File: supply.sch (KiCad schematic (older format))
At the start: 44 parts, among them IC1 MIC5317-2.5YM5-TR, J1 WE_629105150521, U1 FT2232HL-REEL, Y1 KX-7_12,MHz

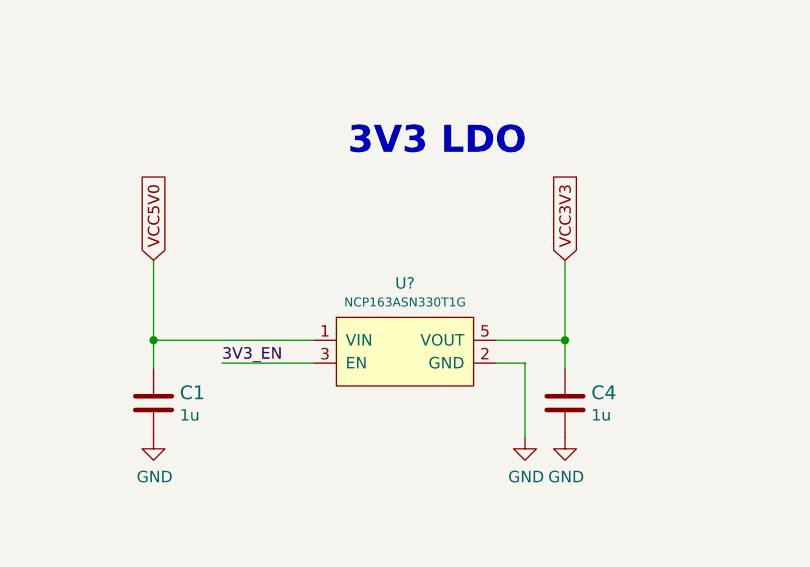
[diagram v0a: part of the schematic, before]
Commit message: Annotate components
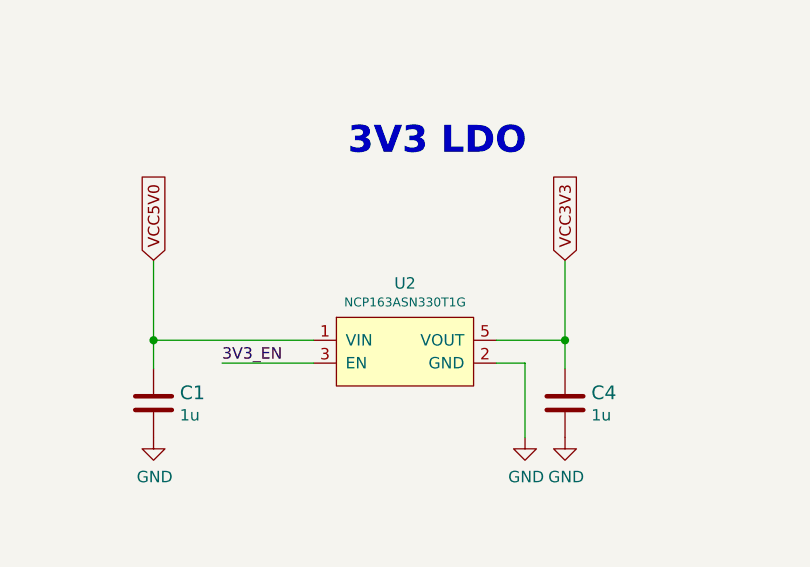
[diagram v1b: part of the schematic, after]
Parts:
- gave numbers to parts that had none: 1
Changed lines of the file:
@@
 VCC3V3
 $Comp
-L rdimm-breakout:NCP163ASN330T1G U?
+L rdimm-breakout:NCP163ASN330T1G U2
 U 1 1 617E4A9E
 P 3100 5875
-F 0 "U?" H 3100 6174 50  0000 C CNN
+F 0 "U2" H 3100 6174 50  0000 C CNN
 F 1 "NCP163ASN330T1G" H 3100 6091 39  0000 C CNN
 F 2 "rdimm-breakout-footprints:SOT-23-5" H 3100 5625 50  0001 C CNN
